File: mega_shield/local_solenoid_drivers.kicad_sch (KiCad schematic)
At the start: 15 parts, among them J18 1803277, J19 1803277, Q23 AO4486, Q24 AO4486, U22 NUP2202

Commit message: mega_shield, changed footprint for AO4486 to use the built in SO-8-8_3.9mmx4.9mm_P1.27mm
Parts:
- Q23, Q24: footprint PCM_Package_SO_AKL:SO-8_3.9x4.9mm_P1.27mm -> Package_SO:SOP-8_3.76x4.96mm_P1.27mm
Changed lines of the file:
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@@
 			)
 		)
-		(property "Footprint" "PCM_Package_SO_AKL:SO-8_3.9x4.9mm_P1.27mm"
+		(property "Footprint" "Package_SO:SOP-8_3.76x4.96mm_P1.27mm"
 			(at 147.32 92.71 0)
 			(effects
@@
 			)
 		)
-		(property "Footprint" "PCM_Package_SO_AKL:SO-8_3.9x4.9mm_P1.27mm"
+		(property "Footprint" "Package_SO:SOP-8_3.76x4.96mm_P1.27mm"
 			(at 205.74 92.71 0)
 			(effects

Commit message: mega_shield, changed footprint for the led to built in 0603(IMPRL)/1608(Metric)
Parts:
- LED8, LED9: footprint PCM_LED_SMD_AKL:LED_0201_0603Metric -> LED_SMD:LED_0603_1608Metric_Pad1.05x0.95mm_HandSolder
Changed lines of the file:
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@@
 			)
 		)
-		(property "Footprint" "PCM_LED_SMD_AKL:LED_0201_0603Metric"
+		(property "Footprint" "LED_SMD:LED_0603_1608Metric_Pad1.05x0.95mm_HandSolder"
 			(at 152.4 57.15 0)
 			(effects
@@
 			)
 		)
-		(property "Footprint" "PCM_LED_SMD_AKL:LED_0201_0603Metric"
+		(property "Footprint" "LED_SMD:LED_0603_1608Metric_Pad1.05x0.95mm_HandSolder"
 			(at 210.82 57.15 0)
 			(effects

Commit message: mega_shield, Changed out all caps where needed for in-stock and lower cost parts.
+ Changed out for parts with higher stock.
+ Changed out for 0805 sized components.
+ Changed out for higher voltage.
+ Removed 22uF SMD caps for lower cost 10uF caps in parallel.
+ Updated diode footprint to SOD-123F

BOM cost reduced, and reliability improved.
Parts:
- D3, D4: footprint PCM_Diode_SMD_AKL:D_SOD-123F -> Diode_SMD:D_SOD-123F
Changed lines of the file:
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@@
 			)
 		)
-		(property "Footprint" "PCM_Diode_SMD_AKL:D_SOD-123F"
+		(property "Footprint" "Diode_SMD:D_SOD-123F"
 			(at 198.12 57.15 0)
 			(effects
@@
 			)
 		)
-		(property "Footprint" "PCM_Diode_SMD_AKL:D_SOD-123F"
+		(property "Footprint" "Diode_SMD:D_SOD-123F"
 			(at 139.7 57.15 0)
 			(effects

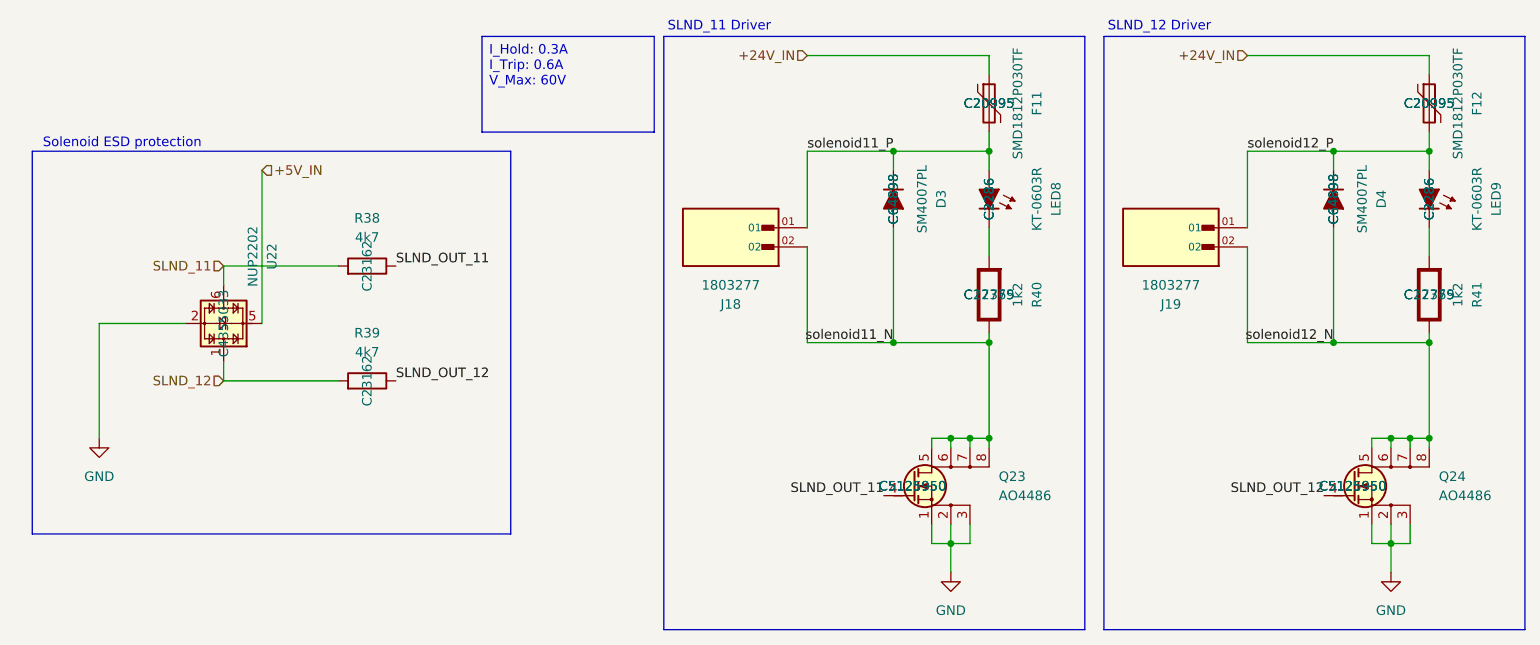
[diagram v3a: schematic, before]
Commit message: mega_shield, updated multiple resistors and added comments.
+ Updated optoisolator resistor value --> 15k for better protection.
+ Changed all resistors to 0805 footprints
+ Swapped out expensive values to standardized E24/E96.
+ Updated jlcpcb numbers for all resistors.
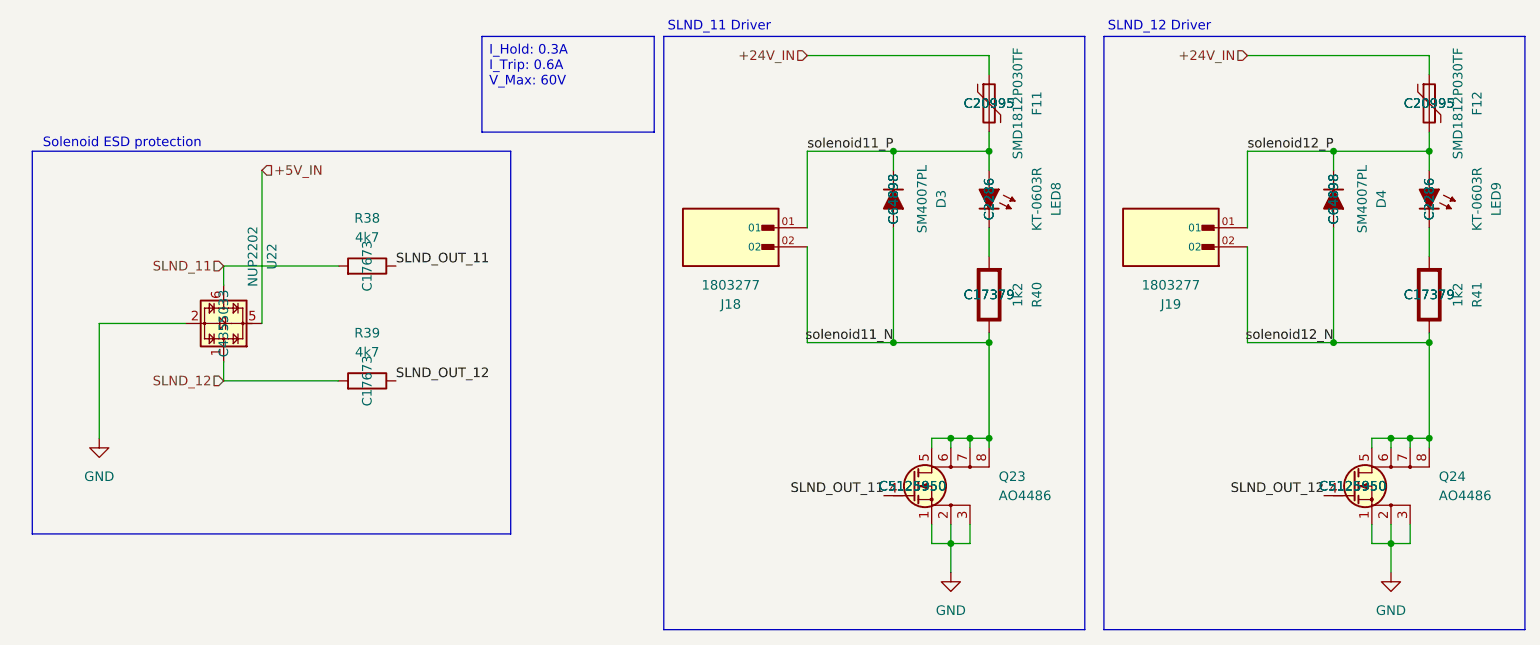
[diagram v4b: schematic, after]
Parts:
- R38, R39: footprint Resistor_SMD:R_0201_0603Metric -> Resistor_SMD:R_0805_2012Metric_Pad1.20x1.40mm_HandSolder; jlcpcb C23162 -> C17673
- R40, R41: footprint Resistor_SMD:R_0201_0603Metric -> Resistor_SMD:R_0805_2012Metric_Pad1.20x1.40mm_HandSolder; jlcpcb C22765 -> C17379
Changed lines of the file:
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@@
 			)
 		)
-		(property "Footprint" "Resistor_SMD:R_0201_0603Metric"
+		(property "Footprint" "Resistor_SMD:R_0805_2012Metric_Pad1.20x1.40mm_HandSolder"
 			(at 69.85 67.818 90)
 			(effects
@@
 			)
 		)
-		(property "jlcpcb" "C23162"
+		(property "jlcpcb" "C17673"
 			(at 69.85 66.04 0)
 			(effects
@@
 			)
 		)
-		(property "Footprint" "Resistor_SMD:R_0201_0603Metric"
+		(property "Footprint" "Resistor_SMD:R_0805_2012Metric_Pad1.20x1.40mm_HandSolder"
 			(at 152.4 69.85 0)
 			(effects
@@
 			)
 		)
-		(property "jlcpcb" "C22765"
+		(property "jlcpcb" "C17379"
 			(at 152.4 69.85 0)
 			(effects
@@
 			)
 		)
-		(property "Footprint" "Resistor_SMD:R_0201_0603Metric"
+		(property "Footprint" "Resistor_SMD:R_0805_2012Metric_Pad1.20x1.40mm_HandSolder"
 			(at 69.85 83.058 90)
 			(effects
@@
 			)
 		)
-		(property "jlcpcb" "C23162"
+		(property "jlcpcb" "C17673"
 			(at 69.85 81.28 0)
 			(effects
@@
 			)
 		)
-		(property "Footprint" "Resistor_SMD:R_0201_0603Metric"
+		(property "Footprint" "Resistor_SMD:R_0805_2012Metric_Pad1.20x1.40mm_HandSolder"
 			(at 210.82 69.85 0)
 			(effects
@@
 			)
 		)
-		(property "jlcpcb" "C22765"
+		(property "jlcpcb" "C17379"
 			(at 210.82 69.85 0)
 			(effects
